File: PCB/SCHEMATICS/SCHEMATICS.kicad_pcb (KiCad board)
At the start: 2 copper layers, 100 x 100 mm, 97 parts, among them IC1 CP2102-GMR, J1 Conn_01x24_Pin, J2 Conn_01x24_Pin, Q1 PMOS, U1 C7433, U2 AMS1117-3.3, U3 LTR-303ALS-01, U4 AMS1117-3.3, U5 LTR-303ALS-01, U6 C6482, U7 C6482

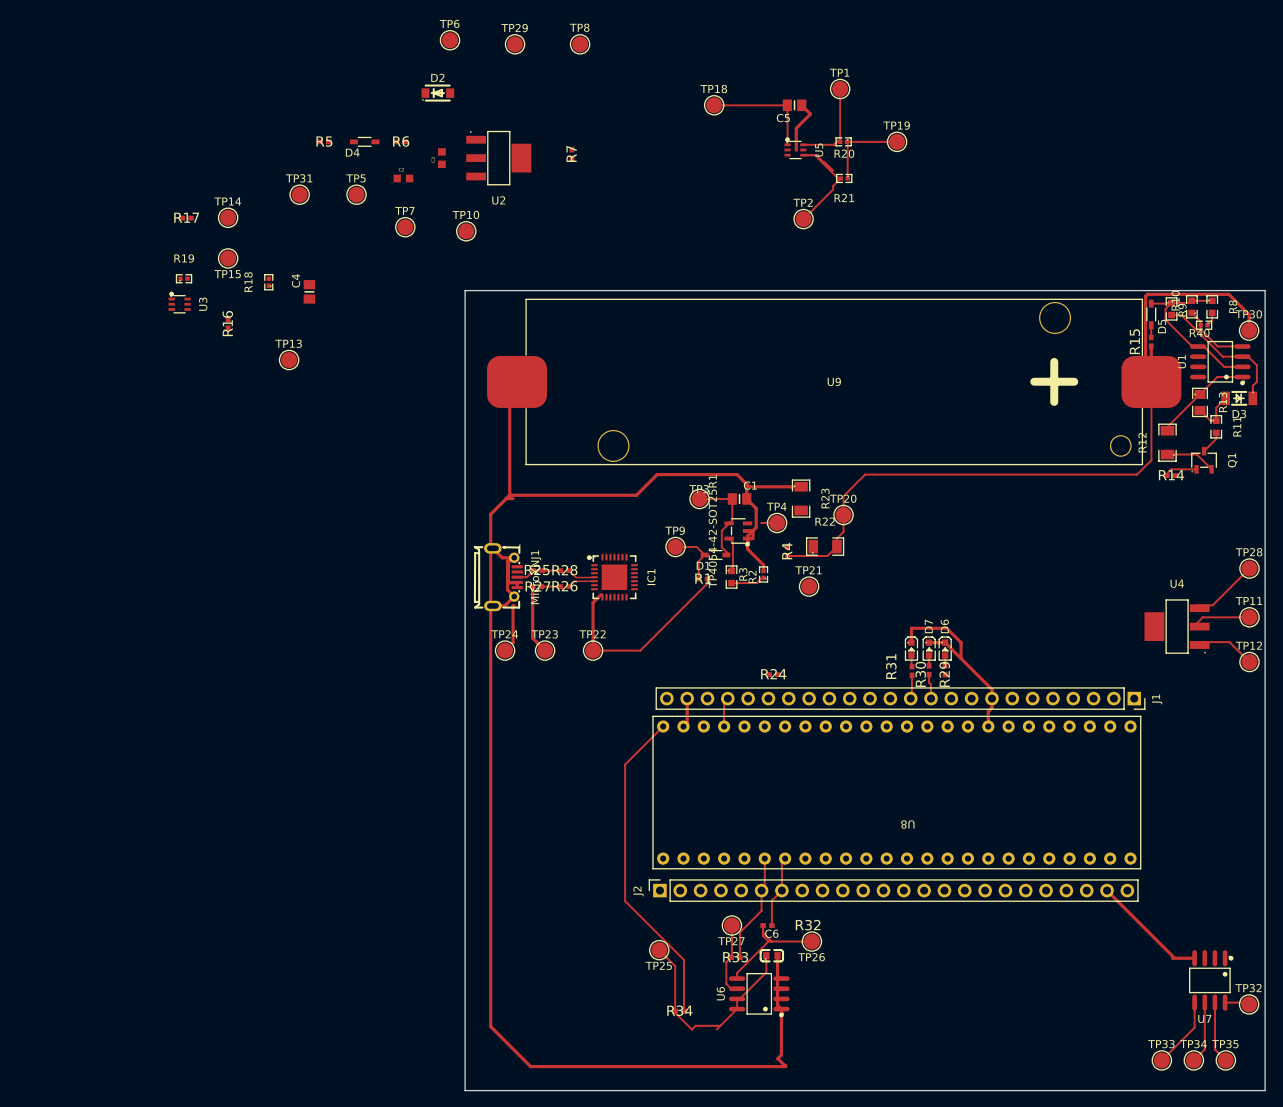
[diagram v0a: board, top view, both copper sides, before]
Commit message: Updated pcb
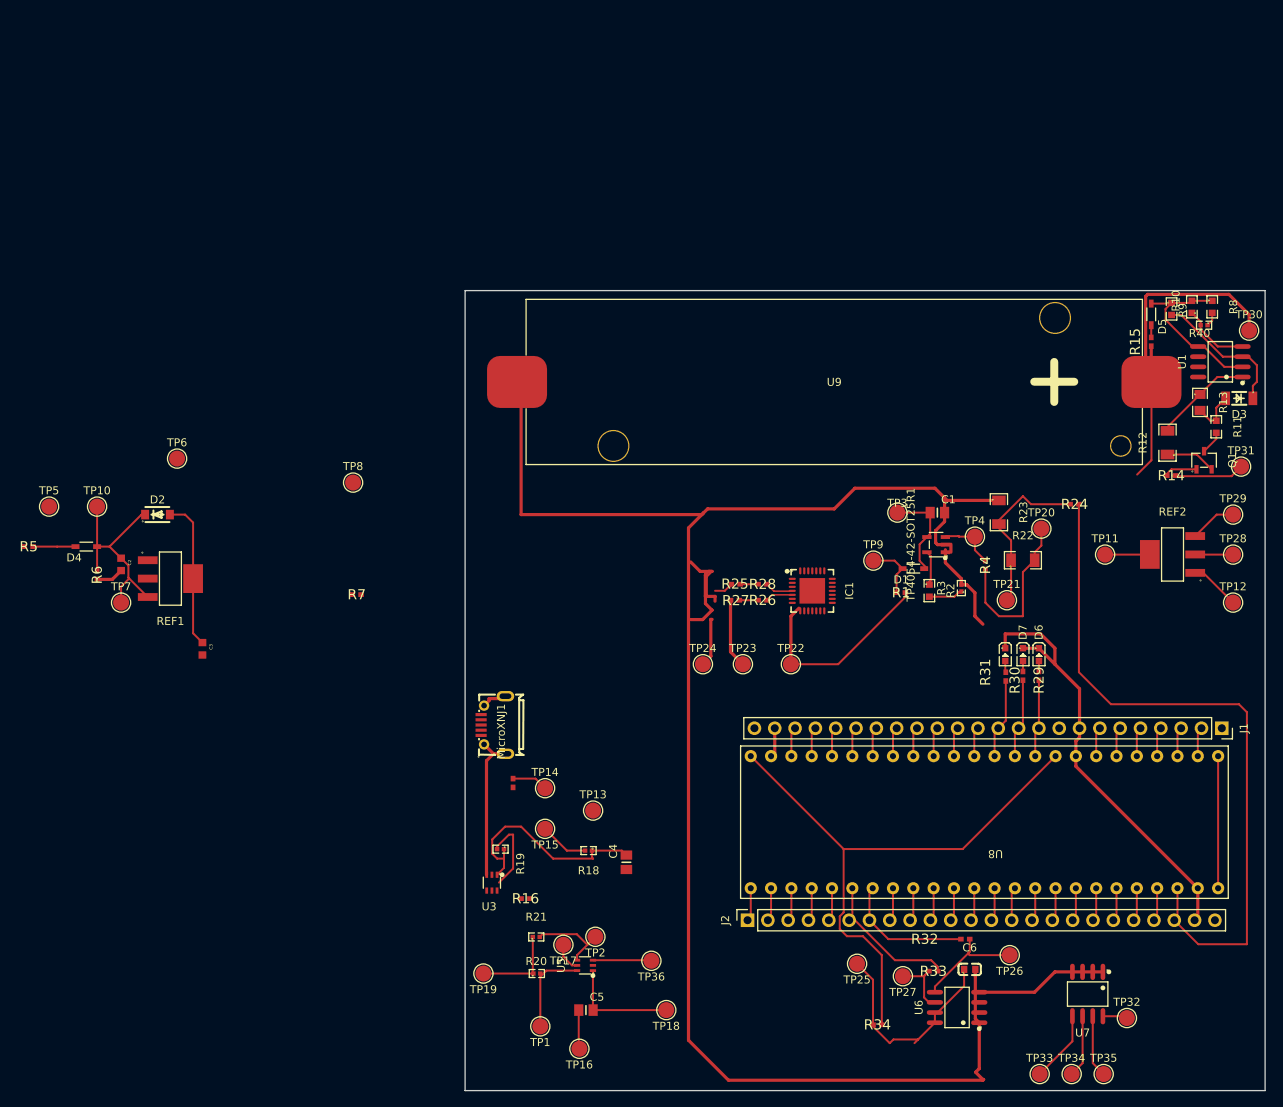
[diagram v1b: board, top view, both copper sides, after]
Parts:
- removed U2, U4: AMS1117-3.3, footprint:SOT-223-4_L6.5-W3.5-P2.30-LS7.0-BR
- added REF1: AMS1117-3_3_C369933, footprint:SOT-223-4_L6.5-W3.5-P2.30-LS7.0-BR, F.Cu at (53.2, 84.0)
- added REF2: AMS1117-3_3_C369933, footprint:SOT-223-4_L6.5-W3.5-P2.30-LS7.0-BR, F.Cu at (178.4, 81.0)
- added TP16: TestPoint, TestPoint:TestPoint_Pad_D2.0mm, F.Cu at (104.3, 142.8)
- added TP17: TestPoint, TestPoint:TestPoint_Pad_D2.0mm, F.Cu at (102.3, 129.8)
- added TP36: TestPoint, TestPoint:TestPoint_Pad_D2.0mm, F.Cu at (113.3, 131.8)
- R40: value 510k -> Value: Value: Value: Value: Value: 510k
- moved TP1 123.0 mm to (99.4, 140.0), turned to 180 degrees
- moved TP31 122.5 mm to (187.0, 70.0)
- moved TP19 116.1 mm to (92.3, 133.4), turned to 180 degrees
- moved C5 116.1 mm to (105.1, 137.9), turned to 0 degrees
- moved TP18 113.3 mm to (115.1, 137.9), turned to 180 degrees
- moved R20 110.8 mm to (99.0, 133.4), turned to 0 degrees
- moved TP29 107.3 mm to (186.0, 76.0)
- moved U5 105.3 mm to (105.0, 132.4), turned to 90 degrees
- moved R21 102.3 mm to (98.9, 128.8), turned to 0 degrees
- moved TP2 93.4 mm to (106.3, 128.8), turned to 180 degrees
- moved U3 82.2 mm to (93.4, 122.0), turned to 180 degrees
- moved TP14 81.6 mm to (100.0, 110.2)
- moved TP15 81.6 mm to (100.0, 115.3)
- moved C4 81.6 mm to (110.2, 119.5)
- moved R17 81.6 mm to (96.0, 109.5), turned to 90 degrees
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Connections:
- C3 pad 1: GND -> Net-(D2-A)
- C5 pad 1: GND -> Net-(C5-Pad1)
- D2 pad 2: GND -> Net-(D2-A)
- R24 pad 2: /MICROCONTROLLER/PA3 -> /MICROCONTROLLER/PB9
- R7 pad 1: GND -> Net-(D2-A)
- TP25 pad : Net-(U6-VCC) -> (no net)
- TP29 pad 1: GND -> Net-(REF2-Input)
- TP6 pad 1: GND -> Net-(D2-A)
- TP8 pad 1: GND -> Net-(D2-A)
- U5 pad 3: GND -> Net-(U5-GND)
- U5 pad 5: GND -> Net-(U5-INT)
- U8 pad 38: /MICROCONTROLLER/PAQ15 -> /MICROCONTROLLER/PA15
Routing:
- net /MICROCONTROLLER/PB9: track 0.00 -> 87.6 mm
- net GND: track 261.9 -> 342.8 mm
- net /MICROCONTROLLER/VSS: track 40.6 -> 117.8 mm
- net /POWER MODULE/Battery: track 95.0 -> 65.4 mm
- net Net-(D2-K): track 0.00 -> 27.4 mm
- net Net-(R22-Pad1): track 0.00 -> 21.5 mm
- net Net-(D2-A): track 0.00 -> 18.8 mm
- net Net-(U3-SCL): track 0.00 -> 14.2 mm
- net /MICROCONTROLLER/PA0: track 0.00 -> 9.68 mm
- net /POWER MODULE/UVLO Output: track 0.43 -> 9.14 mm
- net /MICROCONTROLLER/PA10: track 9.05 -> 16.8 mm
- net Net-(U5-GND): track 0.00 -> 7.34 mm
- net Net-(U5-SCL): track 17.7 -> 10.5 mm
- net /MICROCONTROLLER/PA2: track 2.97 -> 9.97 mm
- net /MICROCONTROLLER/PA1: track 3.10 -> 9.90 mm
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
